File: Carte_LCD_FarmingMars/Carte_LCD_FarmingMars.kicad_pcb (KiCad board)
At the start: 2 copper layers, 22 parts, among them J1 Screw_Terminal_01x02, J2 Conn_01x02_Pin, J3 Conn_01x04_Pin, J4 Conn_01x02_Pin, SW1 SW_DIP_x01, SW2 SW_Push, SW3 SW_Push, U1 3V3 reg, U2 ATtiny1616-S

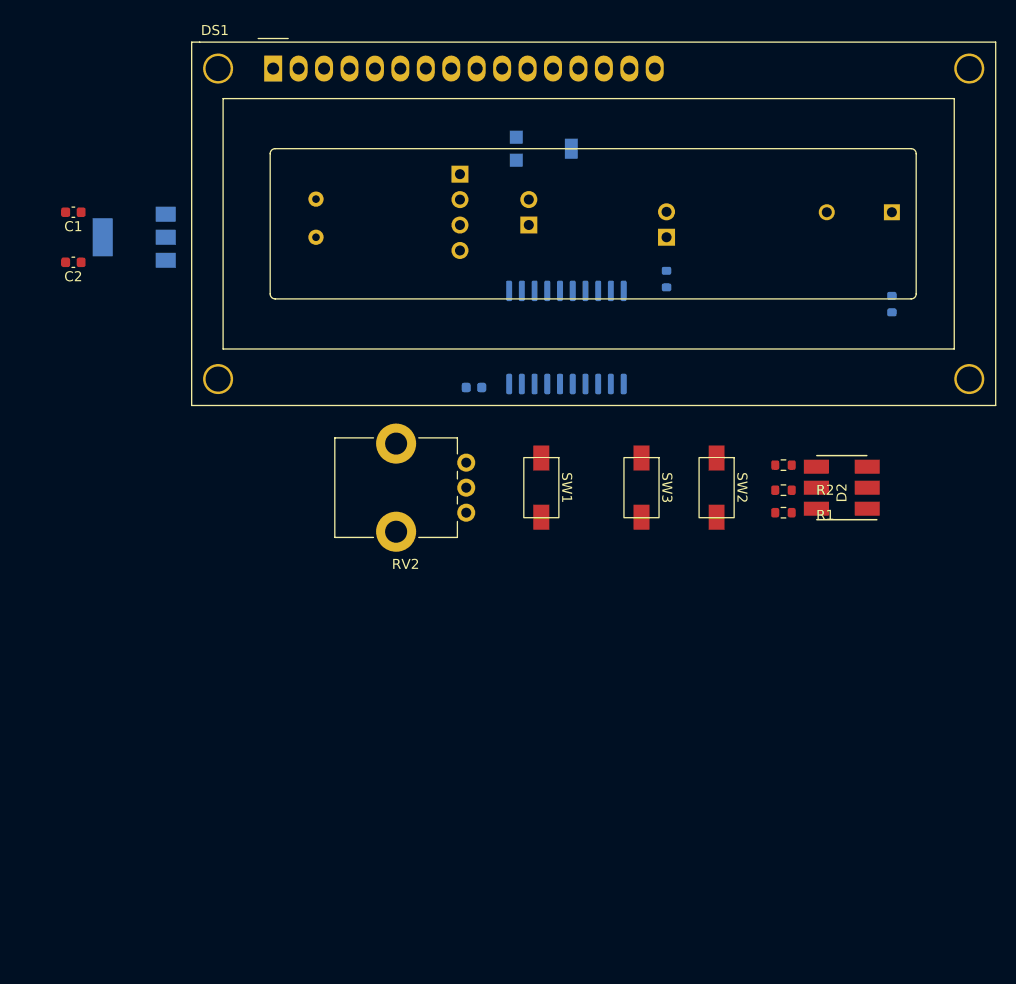
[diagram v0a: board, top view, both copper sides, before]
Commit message: placement composants
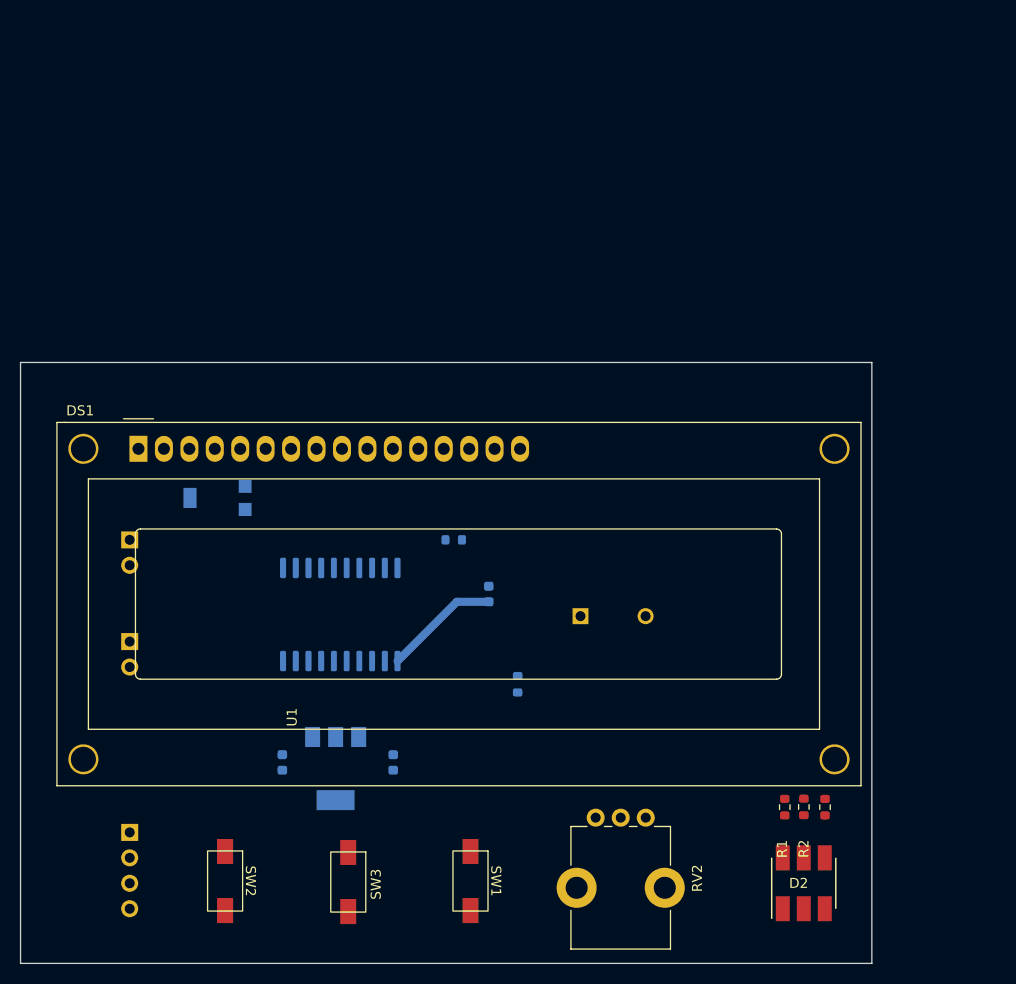
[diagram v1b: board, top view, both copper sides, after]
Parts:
- removed J1: Screw_Terminal_01x02, ENAC_robotique:Bornier_2x3.81mm
- C1, C2: moved to B.Cu
- moved J3 73.5 mm to (88.9, 121.9)
- moved SW2 62.9 mm to (98.4, 126.8)
- moved J4 61.5 mm to (88.9, 92.7), turned to 180 degrees
- moved C2 59.3 mm to (115.2, 114.9), turned to -90 degrees
- moved C1 58.8 mm to (104.1, 114.9), turned to -90 degrees
- moved J2 57.6 mm to (88.9, 102.9), turned to 180 degrees
- moved U1 56.7 mm to (109.5, 115.5), turned to -90 degrees
- moved R_Buzz1 53.3 mm to (127.6, 107.1)
- moved BZ1 50.9 mm to (133.9, 100.3), turned to 0 degrees
- moved SW3 49.1 mm to (110.7, 126.9)
- moved RV1 47.4 mm to (97.9, 88.5), turned to -90 degrees
- moved DS1 40.3 mm to (89.8, 83.6)
- moved SW1 39.9 mm to (122.9, 126.8)
- moved D2 39.7 mm to (156.2, 127.0), turned to 90 degrees
- moved RV2 37.7 mm to (135.4, 120.5), turned to -90 degrees
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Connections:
- C1 pad 1: ALIM 5V -> +5V
- U1 pad 1: ALIM 5V -> +5V
- U2 pad 12: D7 -> D4
- U2 pad 13: D6 -> D5
- U2 pad 14: D5 -> D6
- U2 pad 15: D4 -> D7
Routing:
- net +3.3V: track 0.00 -> 11.6 mm
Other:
- board outline added: 85 x 60 mm
